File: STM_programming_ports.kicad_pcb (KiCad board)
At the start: 2 copper layers, 68.6 x 38.1 mm, 6 parts, among them J1 Conn_ARM_JTAG_SWD_10, J2 Conn_ARM_JTAG_SWD_20, J3 Conn_01x02_Male, J4 Conn_01x04_Female, U1 st-linkv2-clone-port, U2 st-linkv2-clone-port

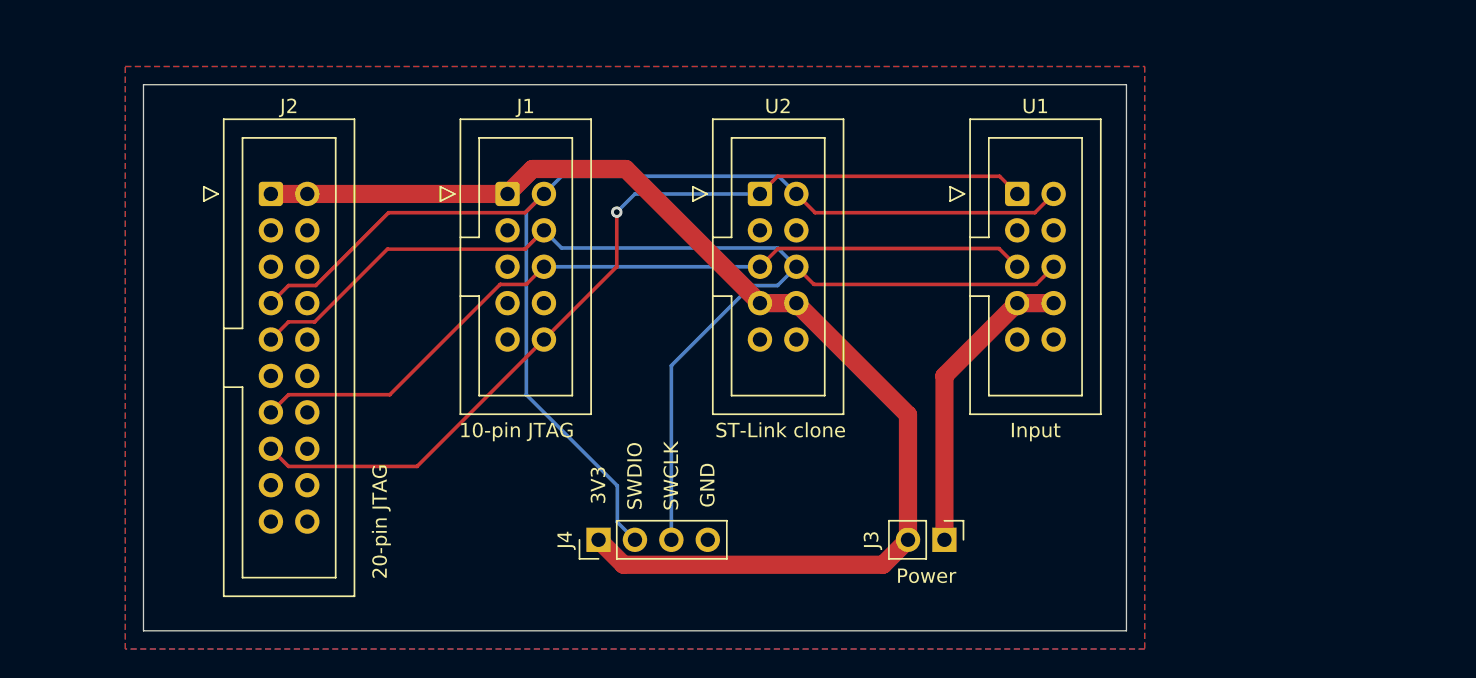
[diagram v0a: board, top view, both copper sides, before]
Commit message: Version02
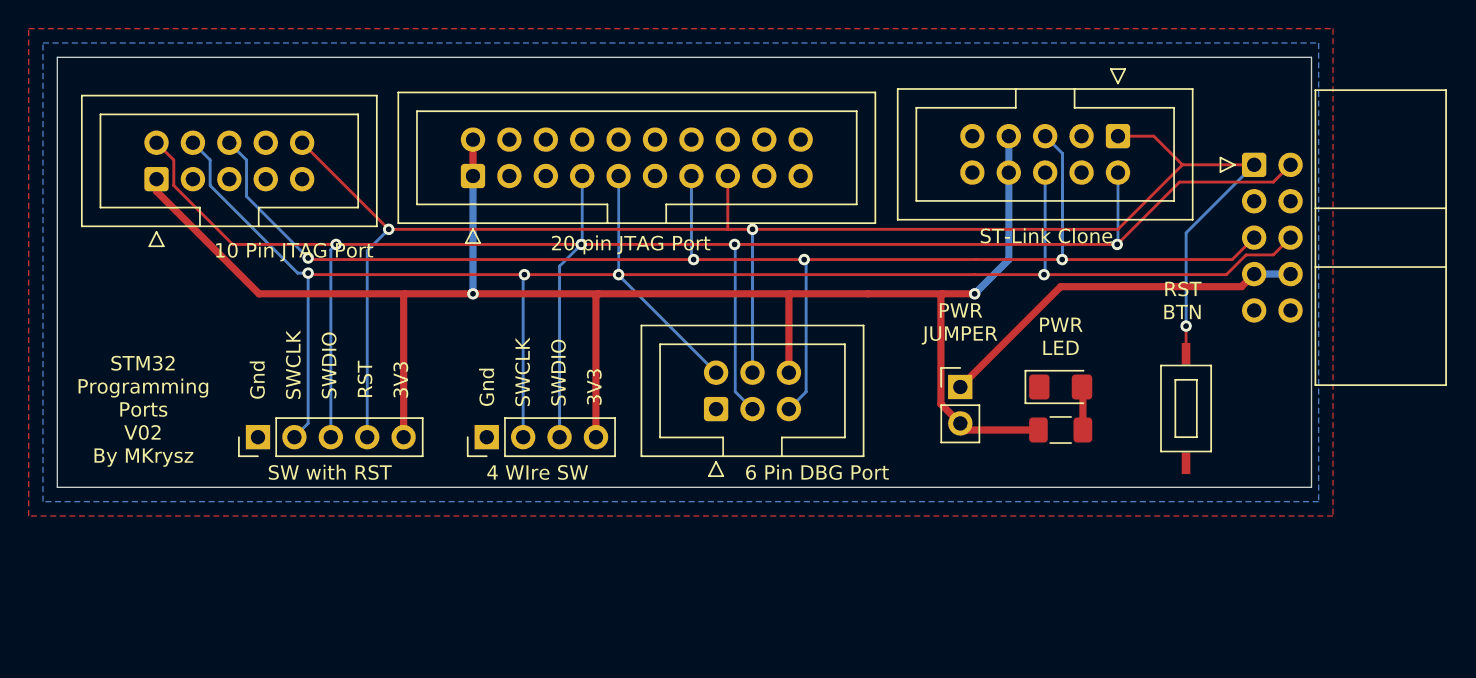
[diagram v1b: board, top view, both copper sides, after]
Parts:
- removed U1, U2: st-linkv2-clone-port, Connector_IDC:IDC-Header_2x05_P2.54mm_Vertical
- added D1: Red, LED_SMD:LED_1206_3216Metric_Pad1.42x1.75mm_HandSolder, F.Cu at (144.0, 63.0)
- added J5: 6PinDebugPort, Connector_IDC:IDC-Header_2x03_P2.54mm_Vertical, F.Cu at (120.0, 64.5)
- added J6: FOUR_WIRE_CONN, Connector_PinHeader_2.54mm:PinHeader_1x04_P2.54mm_Vertical, F.Cu at (104.0, 66.5)
- added J7: st-linkv2-clone-port, Connector_IDC:IDC-Header_2x05_P2.54mm_Vertical, F.Cu at (148.0, 45.5)
- added J8: SW_WITH_RST, Connector_PinHeader_2.54mm:PinHeader_1x05_P2.54mm_Vertical, F.Cu at (88.0, 66.5)
- added R1: 3K9, Resistor_SMD:R_1206_3216Metric_Pad1.30x1.75mm_HandSolder, F.Cu at (144.0, 66.0)
- added SW1: SW_Push, custom_buttons_switches:TSB008, F.Cu at (154.5, 67.5)
- J2: value Conn_ARM_JTAG_SWD_20 -> st-linkv2-clone-port; footprint Connector_IDC:IDC-Header_2x10_P2.54mm_Vertical -> Connector_IDC:IDC-Header_2x05_P2.54mm_Horizontal
- J3: value Conn_01x02_Male -> Conn_ARM_JTAG_SWD_20; footprint Connector_PinHeader_2.54mm:PinHeader_1x02_P2.54mm_Vertical -> Connector_IDC:IDC-Header_2x10_P2.54mm_Vertical
- J4: value Conn_01x04_Female -> Conn_01x02_Male; footprint Connector_PinHeader_2.54mm:PinHeader_1x04_P2.54mm_Vertical -> Connector_PinHeader_2.54mm:PinHeader_1x02_P2.54mm_Vertical
- moved J2 68.6 mm to (157.5, 47.5)
- moved J3 41.5 mm to (103.0, 48.3), turned to 90 degrees
- moved J4 27.4 mm to (137.0, 63.0), turned to 0 degrees
- moved J1 24.5 mm to (80.9, 48.5), turned to 90 degrees
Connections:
- J1 pad 7: Net-(J1-Pad7) -> (no net)
- J1 pad 8: Net-(J1-Pad8) -> (no net)
- J2 pad 1: +3V3 -> /RST
- J2 pad 10: GND -> (no net)
- J2 pad 2: +3V3 -> /SWDIO
- J2 pad 3: Net-(J2-Pad3) -> GND
- J2 pad 5: Net-(J2-Pad5) -> /SWIM
- J2 pad 6: GND -> /SWCLK
- J2 pad 7: /SWDIO -> Net-(J2-Pad7)
- J2 pad 8: GND -> Net-(J2-Pad7)
- J2 pad 9: /SWCLK -> (no net)
- J3 pad 1: Net-(J3-Pad1) -> +3V3
- J4 pad 1: +3V3 -> Net-(J2-Pad7)
- J4 pad 2: /SWDIO -> +3V3
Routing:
- net /RST: track 63.7 -> 120.1 mm, vias 1 -> 3
- net /SWDIO: track 87.7 -> 134.9 mm, vias 0 -> 4
- net /SWCLK: track 83.6 -> 129.6 mm, vias 0 -> 4
- net /SWIM: track 57.3 -> 103.1 mm, vias 0 -> 4
- net +3V3: track 84.0 -> 124.6 mm, vias 0 -> 2
- net Net-(J2-Pad7): track 0.00 -> 26.3 mm
- net Net-(J3-Pad1): track 21.2 -> 0.00 mm
- net Net-(D1-Pad2): track 0.00 -> 3.03 mm
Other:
- board size 68.6 x 38.1 mm -> 87.5 x 30 mm
- board text added: "10 Pin JTAG Port"
- board text added: "20 pin JTAG Port"
- board text added: "4 WIre SW"
- board text added: "6 Pin DBG Port"
- board text added: "Gnd"
- board text added: "JLCJLCJLCJLC"
- board text added: "PWR JUMPER"
- board text added: "PWR LED"
- board text added: "RST"
- board text added: "RST BTN"
- board text added: "ST-Link Clone"
- board text added: "STM32 Programming Ports V02 By MKrysz"
- board text added: "SW with RST"
- board text removed: "10-pin JTAG"
- board text removed: "20-pin JTAG"
- board text removed: "GND"
- board text removed: "Input"
- board text removed: "Power"
- board text removed: "ST-Link clone"
- board text removed: "STM32_programming_ports by MKrysz"
- board text removed: "V01"
